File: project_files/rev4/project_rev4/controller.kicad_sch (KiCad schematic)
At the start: 26 parts, among them J8 USB_C_Receptacle_USB2.0_16P, SW1 JS102011SAQN, SW2 PTS810 SJM 250 SMTR LFS, SW3 PTS810 SJM 250 SMTR LFS, U5 ESP32-S3-WROOM-1-N16R8, U6 AZ1117CH-3.3

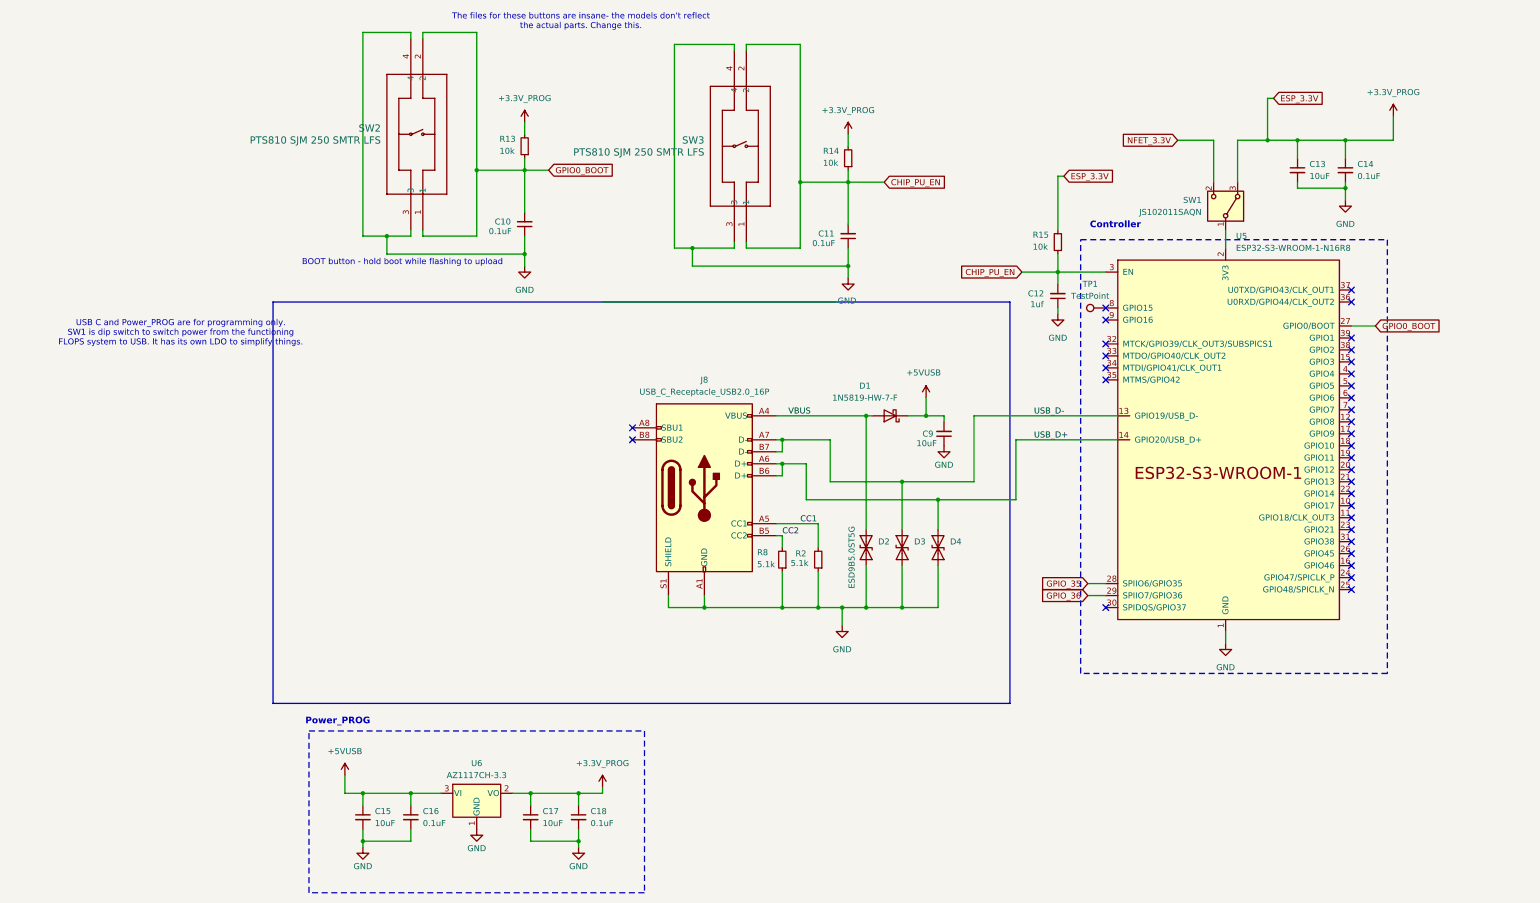
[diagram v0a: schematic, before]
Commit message: committing update
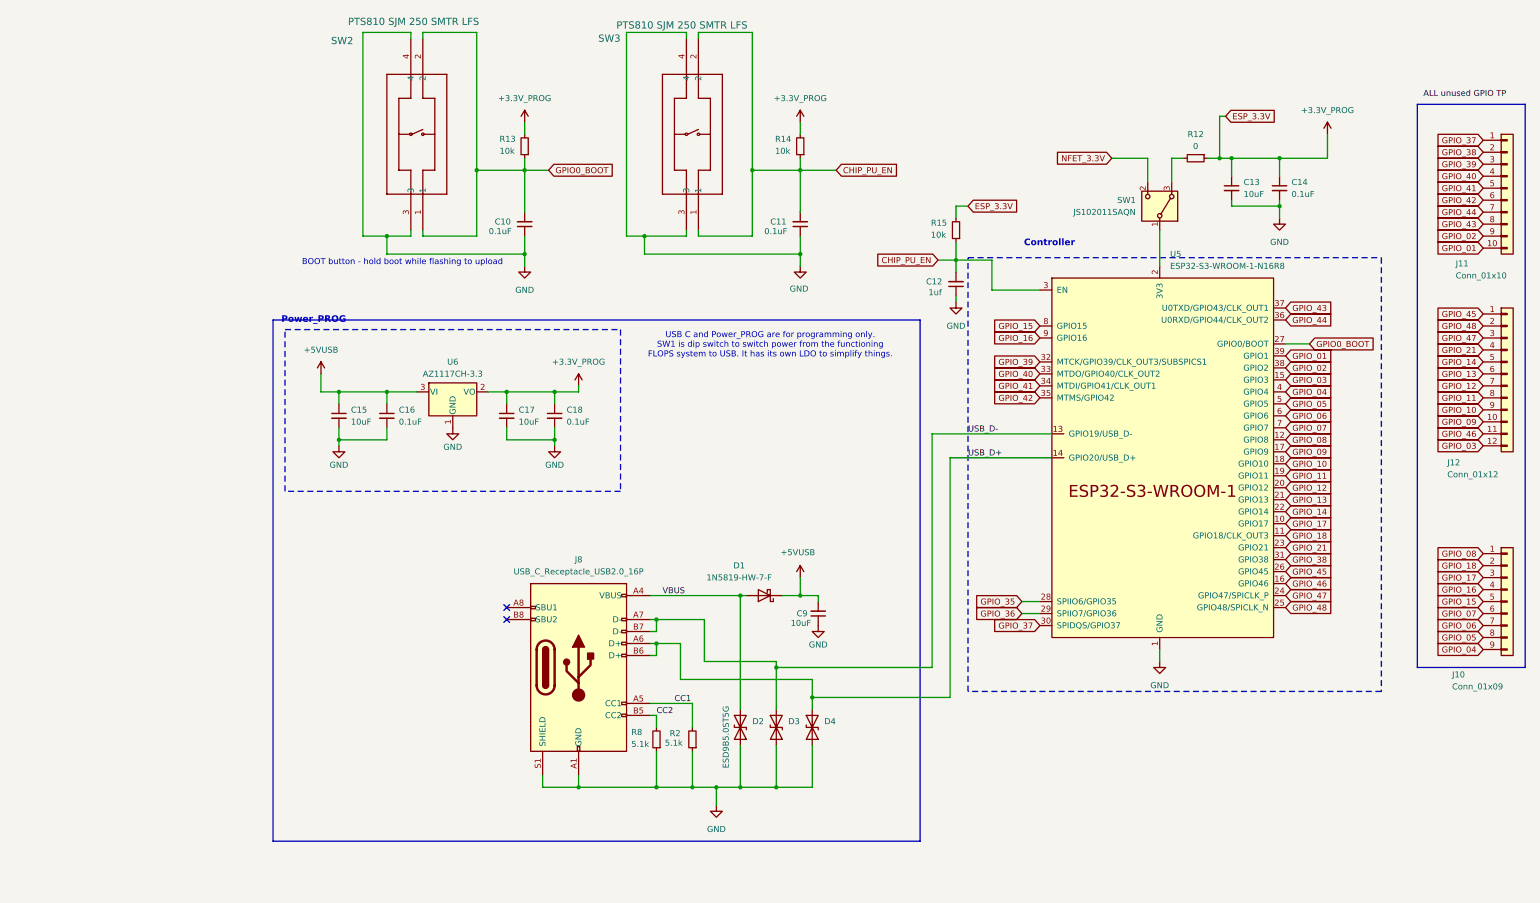
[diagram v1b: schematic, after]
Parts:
- removed TP1: TestPoint, symbol Connector:TestPoint
- added J10: Conn_01x09, Connector_PinHeader_2.54mm:PinHeader_1x09_P2.54mm_Vertical, symbol Connector_Generic:Conn_01x09
- added J11: Conn_01x10, Connector_PinHeader_2.54mm:PinHeader_1x10_P2.54mm_Vertical, symbol Connector_Generic:Conn_01x10
- added J12: Conn_01x12, Connector_PinHeader_2.54mm:PinHeader_1x12_P2.54mm_Vertical, symbol Connector_Generic:Conn_01x12
- added R12: 0, Resistor_SMD:R_0603_1608Metric_Pad0.98x0.95mm_HandSolder, symbol Device:R_Small
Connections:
- net +3.3V_PROG: now also R12.1; no longer SW1.3 (A)
- net GPIO_17: now reaches U5.10 (GPIO17)
- net GPIO_17: now also J10.3 (Pin_3)
- net GPIO_18: now reaches U5.11 (GPIO18/CLK_OUT3)
- net GPIO_18: now also J10.2 (Pin_2)
- net GPIO_08: now reaches U5.12 (GPIO8)
- net GPIO_08: now also J10.1 (Pin_1)
- net GPIO_03: now reaches U5.15 (GPIO3)
- net GPIO_03: now also J12.12 (Pin_12)
- net GPIO_46: now reaches U5.16 (GPIO46)
- net GPIO_46: now also J12.11 (Pin_11)
- net GPIO_09: now reaches U5.17 (GPIO9)
- net GPIO_09: now also J12.10 (Pin_10)
- net GPIO_10: now reaches U5.18 (GPIO10)
- net GPIO_10: now also J12.9 (Pin_9)
- net GPIO_11: now reaches U5.19 (GPIO11)
- net GPIO_11: now also J12.8 (Pin_8)
- net GPIO_12: now reaches U5.20 (GPIO12)
- net GPIO_12: now also J12.7 (Pin_7)
- net GPIO_13: now reaches U5.21 (GPIO13)
- net GPIO_13: now also J12.6 (Pin_6)
- net GPIO_14: now reaches U5.22 (GPIO14)
- net GPIO_14: now also J12.5 (Pin_5)
- net GPIO_21: now reaches U5.23 (GPIO21)
- net GPIO_21: now also J12.4 (Pin_4)
- net GPIO_47: now reaches U5.24 (GPIO47/SPICLK_P)
- net GPIO_47: now also J12.3 (Pin_3)
- net GPIO_48: now reaches U5.25 (GPIO48/SPICLK_N)
- net GPIO_48: now also J12.2 (Pin_2)
- net GPIO_45: now reaches U5.26 (GPIO45)
- net GPIO_45: now also J12.1 (Pin_1)
- net GPIO_37: now reaches U5.30 (SPIDQS/GPIO37)
- net GPIO_37: now also J11.1 (Pin_1)
- net GPIO_38: now reaches U5.31 (GPIO38)
- net GPIO_38: now also J11.2 (Pin_2)
- net GPIO_39: now reaches U5.32 (MTCK/GPIO39/CLK_OUT3/SUBSPICS1)
- net GPIO_39: now also J11.3 (Pin_3)
- net GPIO_40: now reaches U5.33 (MTDO/GPIO40/CLK_OUT2)
- net GPIO_40: now also J11.4 (Pin_4)
- net GPIO_41: now reaches U5.34 (MTDI/GPIO41/CLK_OUT1)
- net GPIO_41: now also J11.5 (Pin_5)
- net GPIO_42: now reaches U5.35 (MTMS/GPIO42)
- net GPIO_42: now also J11.6 (Pin_6)
- net GPIO_44: now reaches U5.36 (U0RXD/GPIO44/CLK_OUT2)
- net GPIO_44: now also J11.7 (Pin_7)
- net GPIO_43: now reaches U5.37 (U0TXD/GPIO43/CLK_OUT1)
- net GPIO_43: now also J11.8 (Pin_8)
- net GPIO_02: now reaches U5.38 (GPIO2)
- net GPIO_02: now also J11.9 (Pin_9)
- net GPIO_01: now reaches U5.39 (GPIO1)
- net GPIO_01: now also J11.10 (Pin_10)
- net GPIO_04: now reaches U5.4 (GPIO4)
- net GPIO_04: now also J10.9 (Pin_9)
- net GPIO_05: now reaches U5.5 (GPIO5)
- net GPIO_05: now also J10.8 (Pin_8)
- net GPIO_06: now reaches U5.6 (GPIO6)
- net GPIO_06: now also J10.7 (Pin_7)
- net GPIO_07: now reaches U5.7 (GPIO7)
- net GPIO_07: now also J10.6 (Pin_6)
- net GPIO_15: now reaches U5.8 (GPIO15)
- net GPIO_15: now also J10.5 (Pin_5)
- net GPIO_16: now reaches U5.9 (GPIO16)
- net GPIO_16: now also J10.4 (Pin_4)
- new net: R12.2, SW1.3 (A)
- no-connect marks 33 -> 2
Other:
- note removed: "The files for these buttons are insane- the models don't reflect the actual parts. Change this."
- moved on the sheet: C11, C12, C13, C14, C15, C16, C17, C18, C9, D1, D2, D3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
